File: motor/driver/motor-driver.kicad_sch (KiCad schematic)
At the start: 61 parts, among them J1 DEBUG, J2 sensors, J3 controller, J4 motor, J5 thermal, J6 external, U2 LM66100DCK, U4 TJA1051TK-3, U5 RP114x, U6 MCT8316Z-Q1, U7 CH32L103F8U6

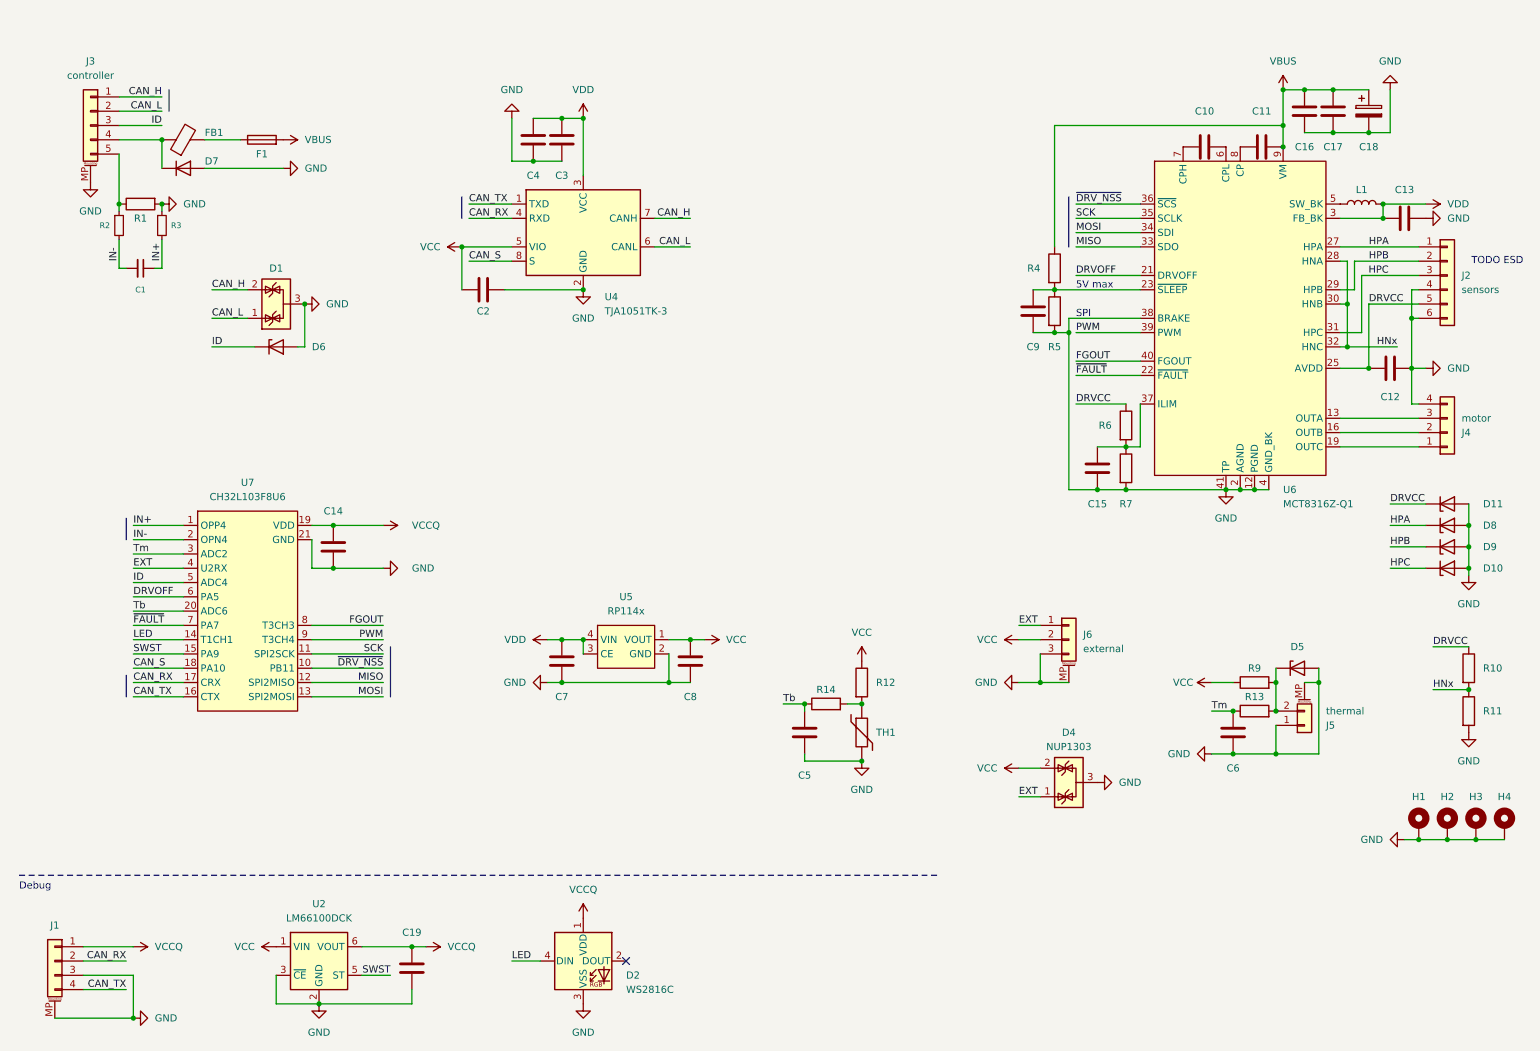
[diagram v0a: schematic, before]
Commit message: driver rev 2
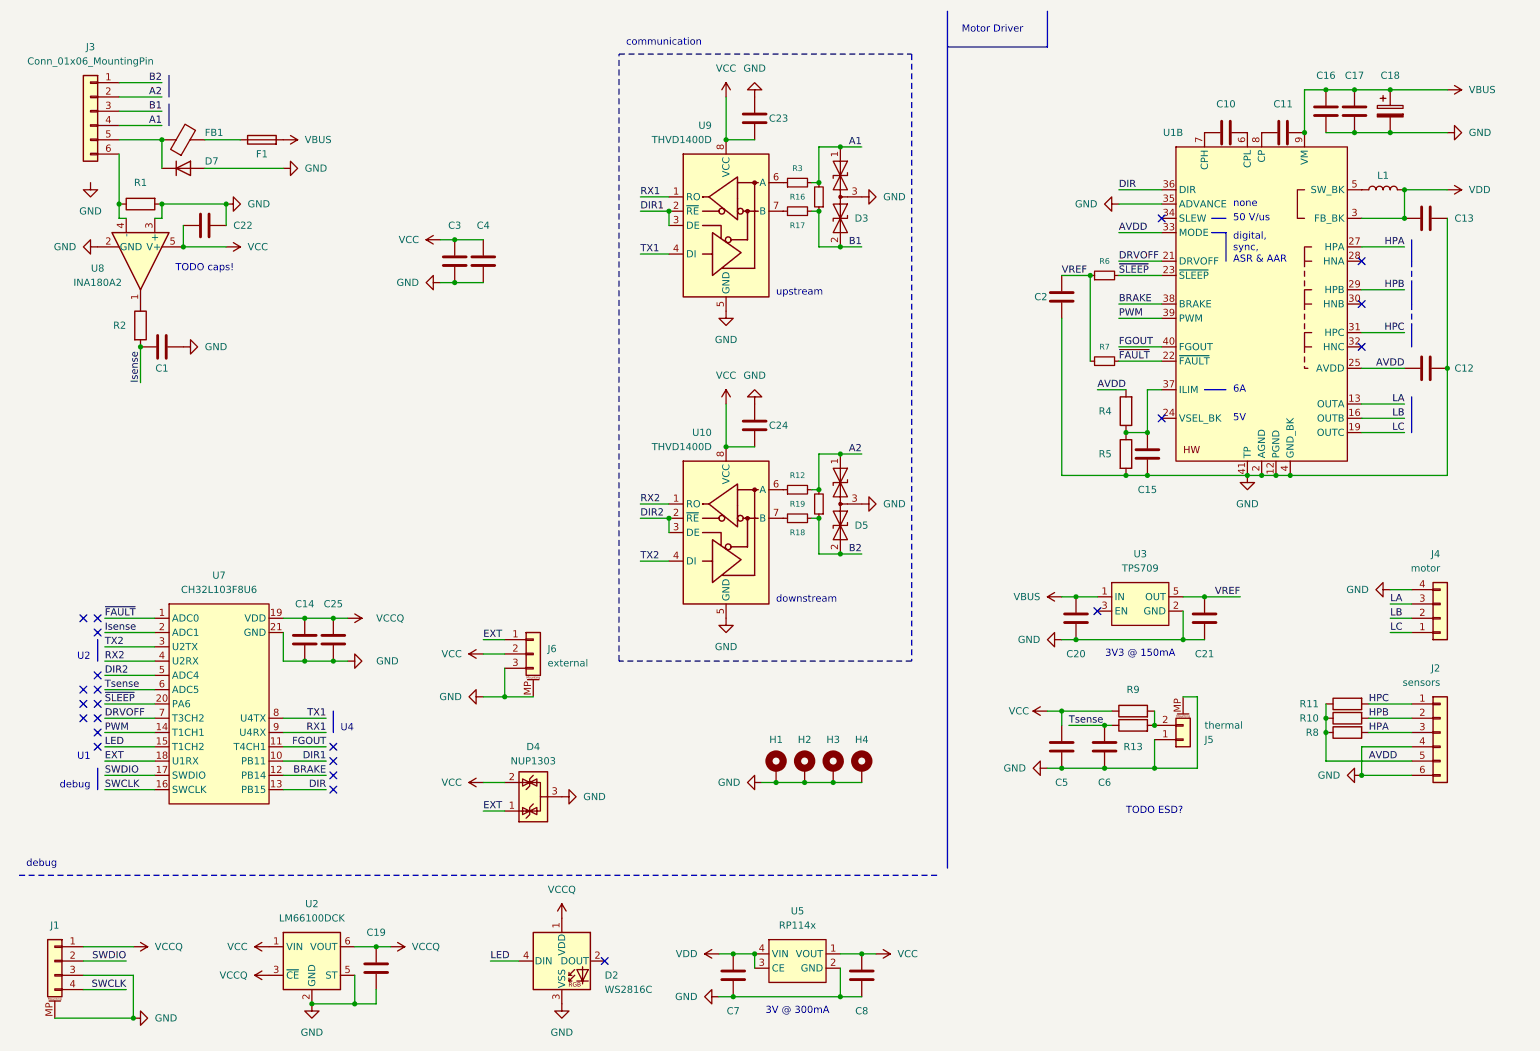
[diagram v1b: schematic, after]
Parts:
- removed C1: 100n, Capacitor_SMD:C_0402_1005Metric, symbol Device:C_Small
- removed C9: 100n, Capacitor_SMD:C_0402_1005Metric, symbol Device:C
- removed D1: SZNUP2105L, Package_TO_SOT_SMD:SOT-23, symbol Power_Protection:SZNUP2105L
- removed D10, D11, D5, D6, D8, D9: PESD5V0L1UL, Diode_SMD:D_SOD-882, symbol Diode:PESD5V0L1UL
- removed J3: controller, Connector_Molex:Molex_Micro-Fit_3.0_43650-0512_1x05-1MP_P3.00mm_Horizontal, symbol Connector_Generic_MountingPin:Conn_01x05_MountingPin
- removed R12, R7: 10k, Resistor_SMD:R_0402_1005Metric, symbol Device:R
- removed R14: 1k, Resistor_SMD:R_0402_1005Metric, symbol Device:R
- removed R2: 10, Resistor_SMD:R_0402_1005Metric, symbol Device:R_Small
- removed R6: 13.7k, Resistor_SMD:R_0402_1005Metric, symbol Device:R
- removed TH1: Thermistor, Resistor_SMD:R_0402_1005Metric, symbol Device:Thermistor
- removed U4: TJA1051TK-3, Package_SON:HVSON-8-1EP_3x3mm_P0.65mm_EP1.6x2.4mm, symbol Interface_CAN_LIN:TJA1051TK-3
- removed U6: MCT8316Z-Q1, misc:QFN-40_EP_5x7_Pitch0.5mm, symbol ti:MCT8316Z-Q1
- added C1: 100n, symbol Device:C
- added C20: 1u, Capacitor_SMD:C_0402_1005Metric, symbol Device:C
- added C21, C25: 2.2u, Capacitor_SMD:C_0402_1005Metric, symbol Device:C
- added C22, C23, C24: 100n, Capacitor_SMD:C_0402_1005Metric, symbol Device:C
- added D3, D5: SM712_SOT23, Package_TO_SOT_SMD:SOT-23, symbol Diode:SM712_SOT23
- added J3: Conn_01x06_MountingPin, Connector_Molex:Molex_Micro-Fit_3.0_43650-0600_1x06_P3.00mm_Horizontal, symbol Connector_Generic:Conn_01x06
- added R12, R16, R17, R18, R19: R_Small, Resistor_SMD:R_0402_1005Metric, symbol Device:R_Small
- added R2: 100, symbol Device:R
- added R6, R7: 5.1k, symbol Device:R_Small
- added R8: 4.7k, Resistor_SMD:R_0402_1005Metric, symbol Device:R
- added U1: MCT8316Z, misc:QFN-40_EP_5x7_Pitch0.5mm, symbol ti:MCT8316Z
- added U10, U9: THVD1400D, Package_TO_SOT_SMD:SOT-583-8, symbol Interface_UART:THVD1400D
- added U3: TPS709, Package_TO_SOT_SMD:SOT-23-5, symbol ti:TPS709
- added U8: INA180A2, Package_TO_SOT_SMD:SOT-23-5, symbol Amplifier_Current:INA180A2
- C10, C16, C17, C18: rating (none) -> VSYS * 2
- C11: rating (none) -> 16V
- C12: rating (none) -> 6.3V
- C13: rating (none) -> VDD * 2
- C15: footprint Capacitor_SMD:C_0402_1005Metric -> (none); LCSC C77020 -> (none)
- C2: LCSC C77020 -> (none)
- C3, C5: value 100n -> 2.2u; LCSC C77020 -> (none)
- C4: LCSC C307418 -> (none)
- R10, R11: LCSC C2906941 -> (none)
- R3: value 10 -> R_Small; LCSC C2906862 -> (none)
- R4: value 47k -> 100k; LCSC C2906872 -> (none)
- R5: value 10k -> 68k; LCSC C2906861 -> (none)
- U5: LCSC C246258 -> C194610
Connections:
- net CAN_S is gone; now on net EXT: U7.18 (PA10)
- net SCK is gone; now on net FGOUT: U7.11 (PB6)
- net DRVOFF: now also U7.7 (PA7), U1.21 (DRVOFF); no longer U7.6 (PA5)
- net EXT: no longer U7.4 (PA3)
- net FGOUT: now also U1.40 (FGOUT); no longer U7.8 (PB0)
- net GND: now also U2.5 (ST), C1.2, C20.2, C21.2, C22.2, C23.1, C24.1, C25.2, D3.3 (common), D5.3 (common), U1.12 (PGND), U1.15 (PGND), U1.18 (PGND), U1.2 (AGND), U1.26 (AGND), U1.35 (ADVANCE), U1.4 (GND_BK), U1.41 (TP), U10.5 (GND), U3.2 (GND), U8.2 (GND), U8.3 (+), U9.5 (GND); no longer R11.2, R3.1, U2.3 (~{CE})
- net HPA: now also J2.3 (Pin_3), R8.2, U1.27 (HPA); no longer J2.1 (Pin_1)
- net HPB: now also R10.2, U1.29 (HPB)
- net HPC: now also J2.1 (Pin_1), R11.2, U1.31 (HPC); no longer J2.3 (Pin_3)
- net LED: now also U7.15 (PA9); no longer U7.14 (PA8)
- net PWM: now also U7.14 (PA8), U1.39 (PWM); no longer U7.9 (PB1)
- net VBUS: now also C20.1, U1.10 (VM), U1.11 (VM), U1.9 (VM), U3.1 (IN); no longer R4.1
- net VCC: now also C3.1, C4.1, C5.1, C22.1, C23.2, C24.2, U10.8 (VCC), U8.5 (V+), U9.8 (VCC); no longer C2.1
- net VCCQ: now also U2.3 (~{CE}), C25.1
- net VDD: now also U1.3 (FB_BK); no longer C3.1, C4.1
- net ~{FAULT}: now also U7.1 (PA0), R7.2, U1.22 (~{FAULT}); no longer U7.7 (PA7)
- net at D7.1 (K), FB1.1: now also J3.5 (Pin_5)
- net LA: now reaches J4.3 (Pin_3)
- net LA: now also U1.13 (OUTA), U1.14 (OUTA)
- net LB: now reaches J4.2 (Pin_2)
- net LB: now also U1.16 (OUTB), U1.17 (OUTB)
- net LC: now reaches J4.1 (Pin_1)
- net LC: now also U1.19 (OUTC), U1.20 (OUTC)
- net at R5.1: now also C15.1, R4.1, U1.37 (ILIM); no longer R4.2
- net at L1.1: now also U1.5 (SW_BK)
- net at C10.2: now also U1.6 (CPL)
- net at C10.1: now also U1.7 (CPH)
- net at C11.1: now also U1.8 (CP)
- net at R1.1: now also J3.6 (Pin_6), U8.4 (-)
- net CAN_RX renamed SWDIO
- net CAN_TX renamed SWCLK
- net DRVCC renamed AVDD
- net AVDD: now also R11.1, R4.2, R8.1, U1.25 (AVDD), U1.33 (MODE)
- removed net HNx: R10.2, R11.1
- net ID renamed DIR2
- net DIR2: now also U10.2 (~{RE}), U10.3 (DE)
- net IN+ renamed A1
- net A1: now also D3.1 (A1), J3.4 (Pin_4), R16.2; no longer U7.1 (PA0)
- net IN- renamed Isense
- net Isense: now also C1.1, R2.2
- net MISO renamed BRAKE
- net BRAKE: now also U1.38 (BRAKE)
- net MOSI renamed DIR
- net DIR: now also U1.36 (DIR)
- removed net SWST: U2.5 (ST), U7.15 (PA9)
- net Tb renamed ~{SLEEP}
- net ~{SLEEP}: now also R6.2, U1.23 (~{SLEEP}); no longer C5.1
- net Tm renamed Tsense
- net Tsense: now also U7.6 (PA5); no longer U7.3 (PA2)
- net ~{DRV_NSS} renamed DIR1
- net DIR1: now also U9.2 (~{RE}), U9.3 (DE)
- new net: R3.1, U9.6 (A)
- new net: R18.1, U10.7 (B)
- new net: R12.1, U10.6 (A)
- new net: R17.1, U9.7 (B)
- new net: R2.1, U8.1
- new net A2: D5.1 (A1), J3.2 (Pin_2), R12.2, R19.2
- new net B1: D3.2 (A2), J3.3 (Pin_3), R16.1, R17.2
- new net B2: D5.2 (A2), J3.1 (Pin_1), R18.2, R19.1
- new net RX1: U7.9 (PB1), U9.1 (RO)
- new net RX2: U10.1 (RO), U7.4 (PA3)
- new net TX1: U7.8 (PB0), U9.4 (DI)
- new net TX2: U10.4 (DI), U7.3 (PA2)
- new net VREF: C2.1, C21.1, R6.1, R7.1, U3.5 (OUT)
- no-connect marks 1 -> 23
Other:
- note added: "3V @ 300mA"
- note added: "3V3 @ 150mA"
- note added: "50 V/us"
- note added: "5V"
- note added: "6A"
- note added: "Motor Driver"
- note added: "TODO ESD?"
- note added: "TODO caps!"
- note added: "U1"
- note added: "U2"
- note added: "U4"
- note added: "communication"
- note added: "debug"
- note added: "digital, sync, ASR & AAR"
- note added: "downstream"
- note added: "none"
- note added: "upstream"
- note removed: "5V max"
- note removed: "Debug"
- note removed: "SPI"
- note removed: "TODO ESD"
- moved on the sheet: C10, C11, C14, C16, C17, C18, C19, C6, C7, C8, D2, D4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
